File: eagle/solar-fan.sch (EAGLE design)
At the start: 40 parts, among them J1 POWER_JACKPTH, J2 USB-A-S, J3 7805, U1 LT3652, U2 ATTINY85

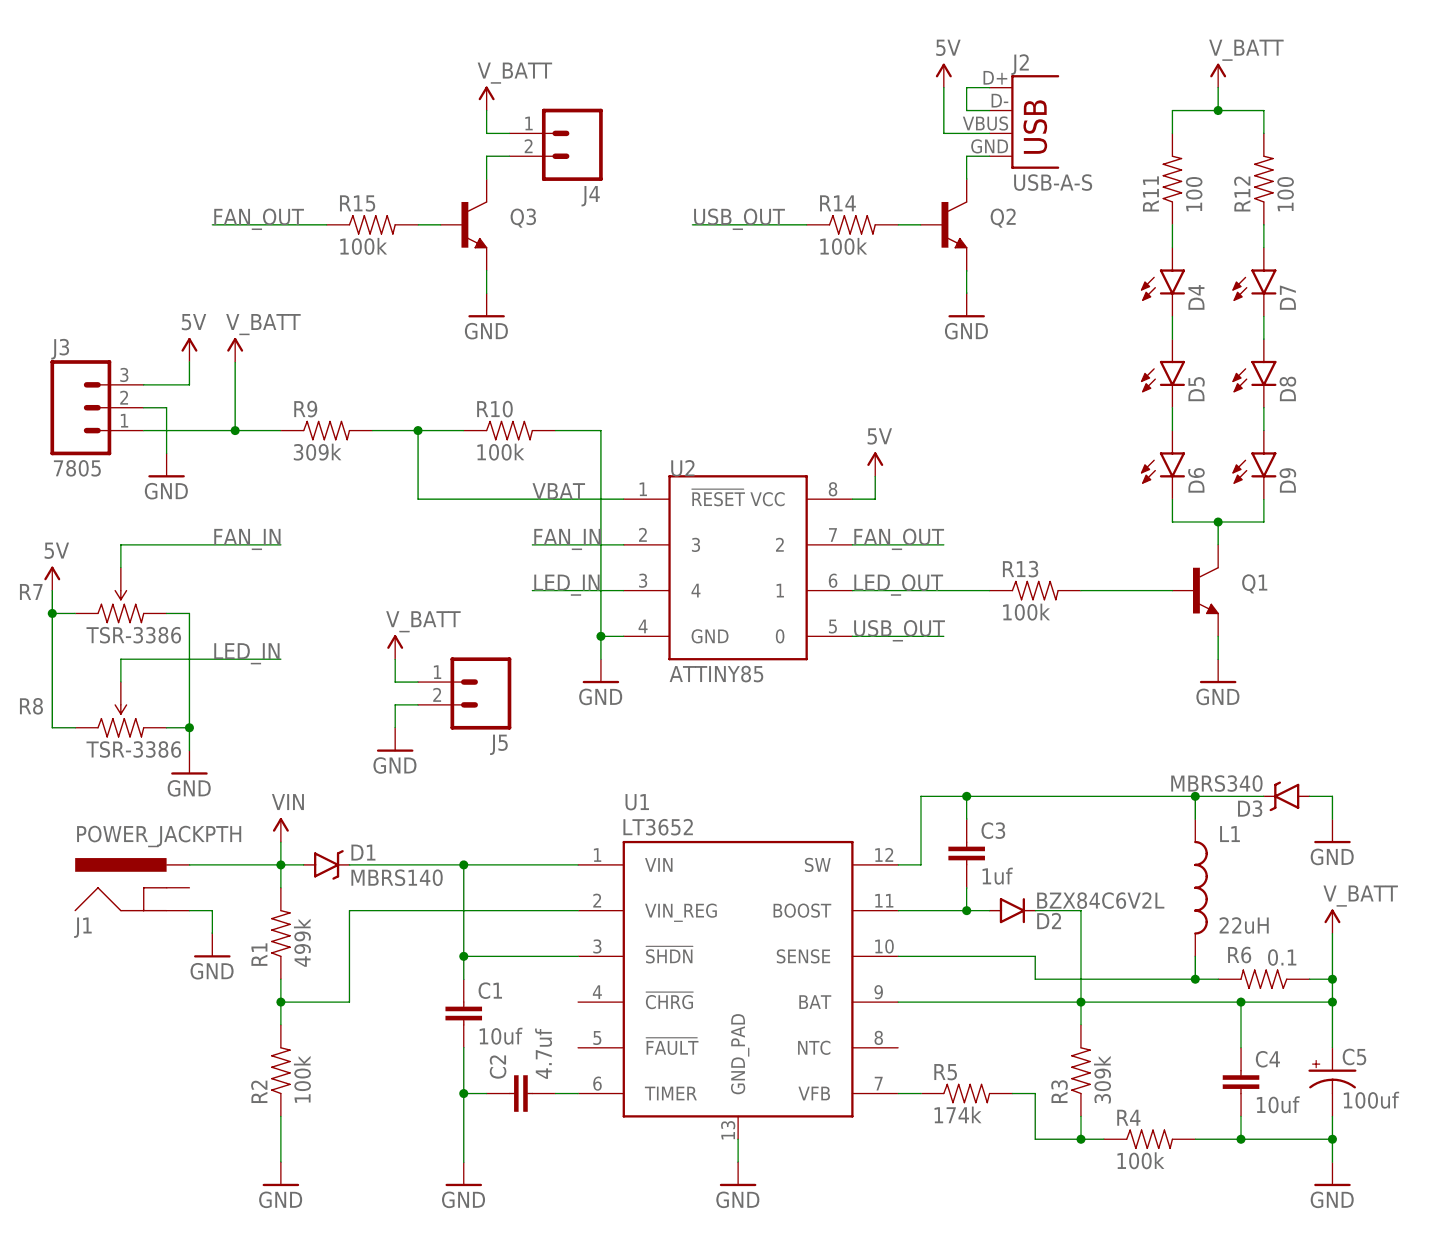
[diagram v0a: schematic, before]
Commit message: layout update, bom, components
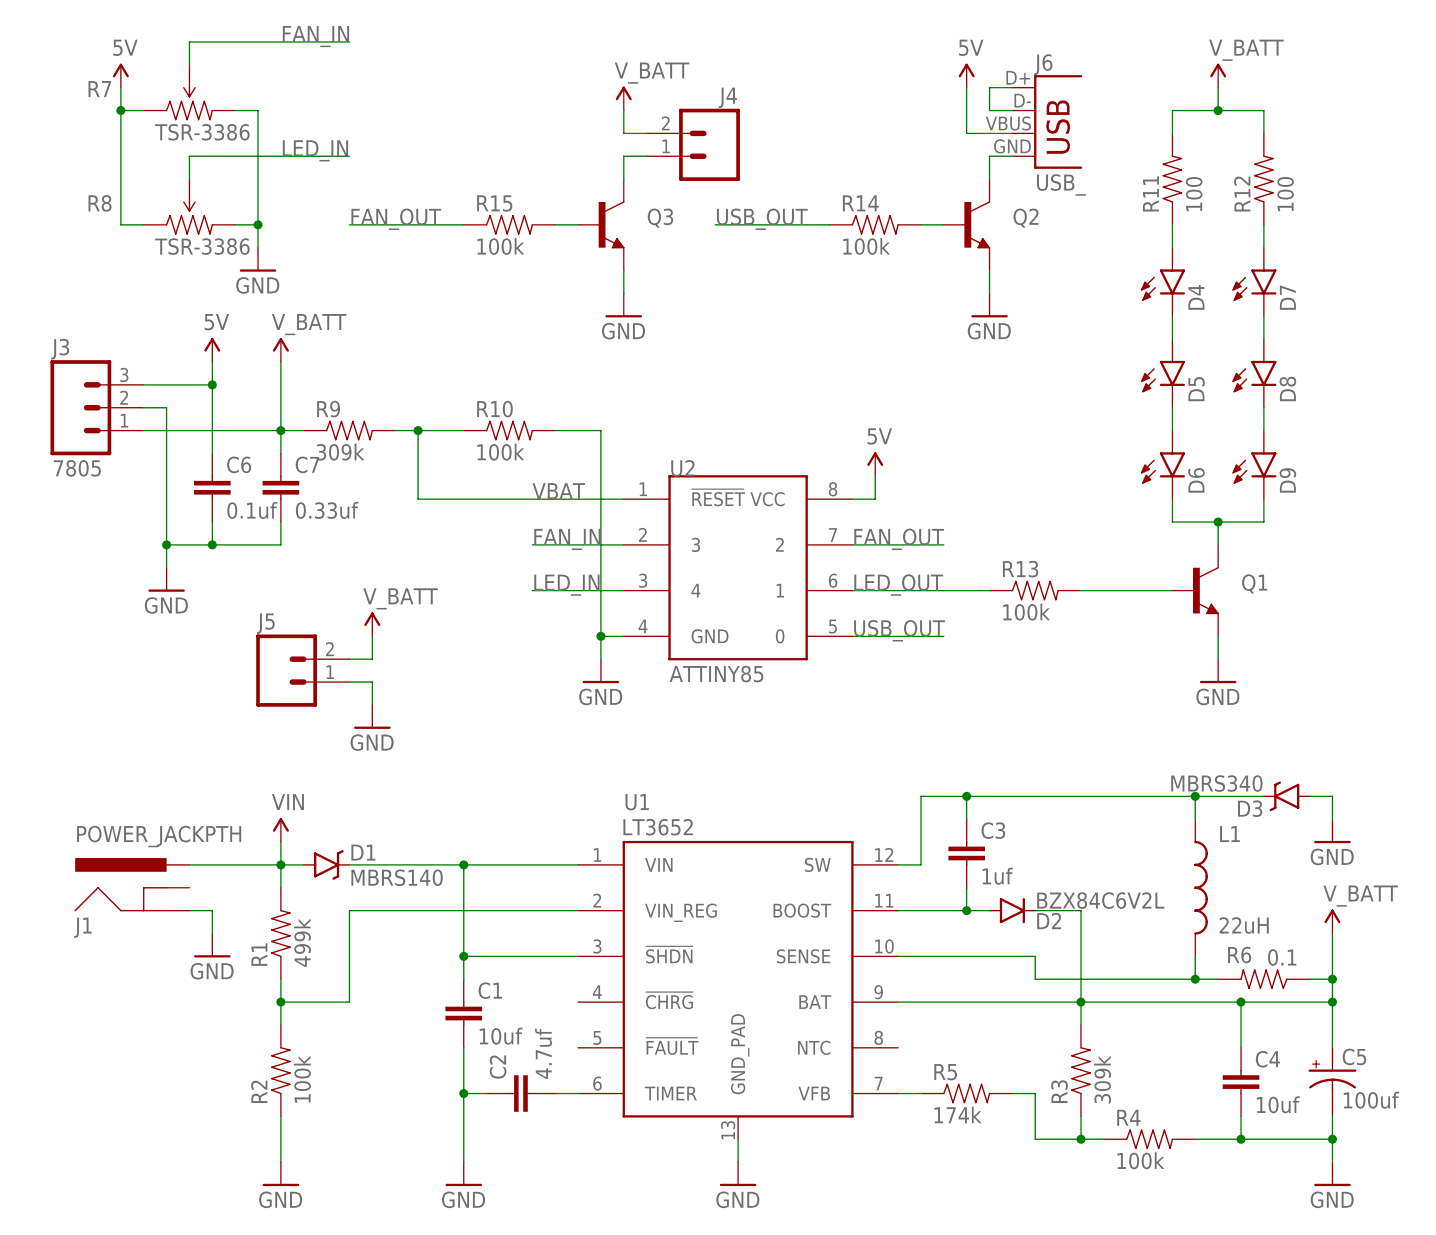
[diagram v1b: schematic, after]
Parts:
- removed J2: USB-A-S, SparkFun-Connectors:USB-A-S
- added C6: 0.1uf, SparkFun-Passives:CAP0603-CAP
- added C7: 0.33uf, SparkFun-Passives:CAP0603-CAP
- added J6: USB_, SparkFun-Connectors:USB_
- C1, C4: PN (none) -> 490-1880-1-ND
- C2: PN (none) -> 490-10481-1-ND
- C3: PN (none) -> 490-1536-1-ND
- C5: PN (none) -> 399-6650-1-ND
- D1: PN MBRS140FSCT-ND -> MBRS140T3GOSCT-ND
- D2: PN (none) -> SZBZX84C6V2LT1GOSCT-ND
- D3: PN (none) -> MBRS340T3GOSTR-ND
- D4, D5, D6, D7, D8, D9: PN 516-2236-1-ND -> 1516-1057-1-ND
- J3: PN (none) -> LM7805CT-ND
- J4: PN (none) -> WM4200-ND
- J5: PN (none) -> 455-1719-ND
- L1: PN (none) -> RLB0912-220KL-ND
- R3: PN (none) -> P309KHCT-ND
- R6: PN (none) -> 1276-6155-1-ND
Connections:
- removed net N$22: J4.2, Q3.C
- new net N$6: J4.1, Q3.C
- net 5V: now also C6.1, J6.VBUS; no longer J2.VBUS
- net GND: now also C6.2, C7.2, J5.1; no longer J5.2
- net N$20: now also J6.D+, J6.D-; no longer J2.D+, J2.D-
- net N$21: now also J6.GND; no longer J2.GND
- net V_BATT: now also C7.1, J4.2, J5.2; no longer J4.1, J5.1
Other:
- moved on the sheet: J4, J5, Q2, Q3, R14, R15, R7, R8, R9
